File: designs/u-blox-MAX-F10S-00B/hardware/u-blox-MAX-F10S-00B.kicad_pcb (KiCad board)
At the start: 2 copper layers, 30 x 30 mm, 13 parts, among them IC101 MAX-F10S-00B, J105 Conn_Coaxial_Small, J106 Conn_Coaxial_Small, U101 MIC5318YMT-TR

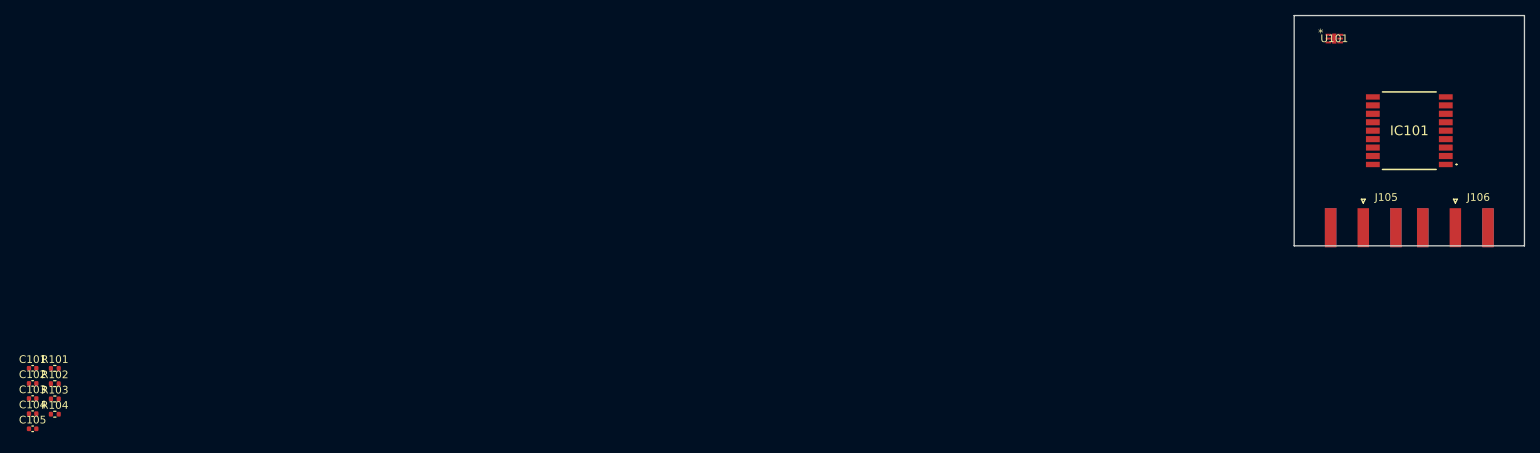
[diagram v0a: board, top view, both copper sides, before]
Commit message: need to check pad to pad clearance of jlcpcb
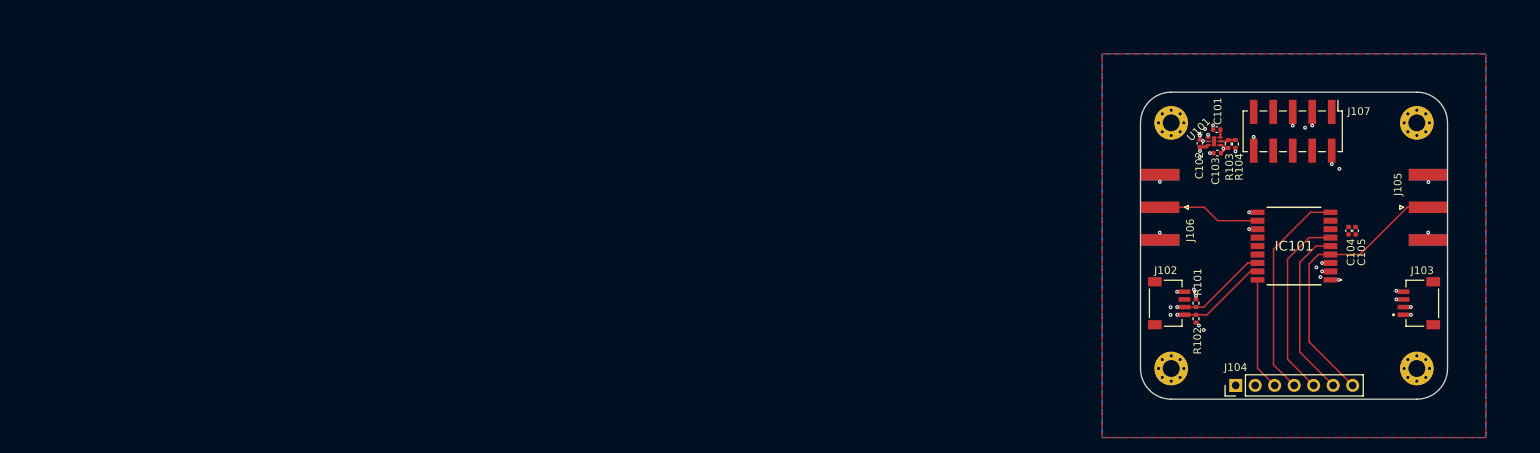
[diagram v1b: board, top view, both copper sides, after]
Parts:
- added H101: MountingHole_Pad, MountingHole:MountingHole_2.2mm_M2_Pad_Via, F.Cu at (134.0, 84.0)
- added H102: MountingHole_Pad, MountingHole:MountingHole_2.2mm_M2_Pad_Via, F.Cu at (166.0, 84.0)
- added H103: MountingHole_Pad, MountingHole:MountingHole_2.2mm_M2_Pad_Via, F.Cu at (134.0, 116.0)
- added H104: MountingHole_Pad, MountingHole:MountingHole_2.2mm_M2_Pad_Via, F.Cu at (166.0, 116.0)
- added J102: PRT-14417, pcb-SparkFun:PRT-14417, F.Cu at (133.3, 107.5)
- added J103: PRT-14417, pcb-SparkFun:PRT-14417, F.Cu at (166.7, 107.5)
- added J104: Conn_01x07_Pin, Connector_PinHeader_2.54mm:PinHeader_1x07_P2.54mm_Vertical, F.Cu at (142.4, 118.2)
- added J107: Conn_02x05_Counter_Clockwise, Connector_PinHeader_2.54mm:PinHeader_2x05_P2.54mm_Vertical_SMD, F.Cu at (149.8, 85.1)
- moved C105 174.3 mm to (158.0, 98.0), turned to -90 degrees
- moved C104 173.1 mm to (157.1, 98.0), turned to -90 degrees
- moved R104 157.8 mm to (142.3, 86.7), turned to -90 degrees
- moved C103 157.6 mm to (140.0, 87.9), turned to 180 degrees
- moved C101 157.4 mm to (139.9, 84.9), turned to 180 degrees
- moved R103 156.4 mm to (141.4, 86.7), turned to 90 degrees
- moved C102 155.3 mm to (137.7, 86.6), turned to 90 degrees
- moved R101 148.9 mm to (137.2, 107.5), turned to -90 degrees
- moved R102 148.9 mm to (137.2, 109.5), turned to 90 degrees
- moved J106 38.6 mm to (132.5, 95.0), turned to 180 degrees
- moved IC101 21.2 mm to (150.0, 100.0)
- moved U101 20.6 mm to (139.6, 86.4)
- moved J105 8.87 mm to (167.5, 95.0), turned to 0 degrees
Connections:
- U101 pad 7: (no net) -> GND
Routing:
- net /SCL: track 0.00 -> 49.5 mm, vias 0 -> 2
- net /SDA: track 0.00 -> 49.4 mm, vias 0 -> 2
- net /TIMEPULSE: track 0.00 -> 36.8 mm
- net /RESET_N: track 0.00 -> 28.3 mm
- net /V_BCKP: track 0.00 -> 24.6 mm
- net /EXTINT: track 0.00 -> 22.7 mm
- net /RXD: track 0.00 -> 21.3 mm, vias 0 -> 2
- net /TXD: track 0.00 -> 21.2 mm, vias 0 -> 2
- net /SAFEBOOT_N: track 0.00 -> 14.7 mm
- net /RF_IN: track 0.00 -> 13.5 mm
- net +3V3: track 0.00 -> 4.10 mm, vias 0 -> 4
- net +5V: track 0.00 -> 3.86 mm, vias 0 -> 3
- net Net-(U101-ADJ): track 0.00 -> 2.08 mm
- net Net-(U101-BYP): track 0.00 -> 1.05 mm
- net GND: vias 0 -> 25
- added copper zone on In2.Cu, net +3V3
- added copper zone on In2.Cu, net +5V
- added copper zone on B.Cu, net GND
- added copper zone on F.Cu, net GND
- added copper zone on In1.Cu, net GND
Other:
- board size 30 x 30 mm -> 40 x 40 mm
- copper layers 2 -> 4
- board text removed: "CHECK MOTOR DRIVER PCB FOR GETTING STARTED...."
